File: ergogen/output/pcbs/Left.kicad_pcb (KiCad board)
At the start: 2 copper layers, 130.3 x 105.3 mm, 44 parts

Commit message: fix xiao footprint
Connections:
- MCU1 pad 17: GND -> RST
- MCU1 pad 18: RST -> GND
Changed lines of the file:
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@@
   (net 15 "DIO"))
   (pad "17" thru_hole circle (at -1.27 -6.032 90) (size 1.397 1.397) (drill 1.016) (layers "*.Cu" "*.Mask")
+  (net 17 "RST"))
+  (pad "18" thru_hole circle (at 1.27 -6.032 90) (size 1.397 1.397) (drill 1.016) (layers "*.Cu" "*.Mask")
   (net 16 "GND"))
-  (pad "18" thru_hole circle (at 1.27 -6.032 90) (size 1.397 1.397) (drill 1.016) (layers "*.Cu" "*.Mask")
-  (net 17 "RST"))
   (pad "19" thru_hole circle (at -4.445 -0.317 180) (size 1.397 1.397) (drill 1.016) (layers "*.Cu" "*.Mask")
   (net 18 "BAT"))

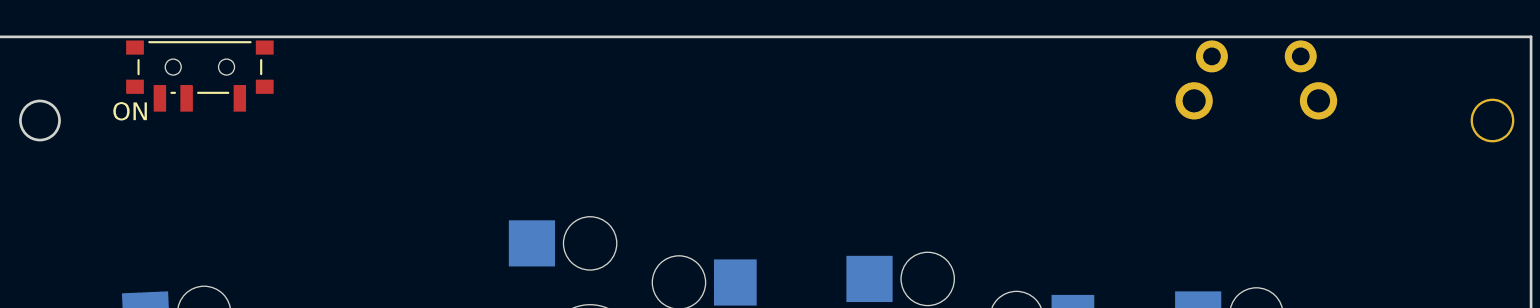
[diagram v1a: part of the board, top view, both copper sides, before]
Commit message: update config
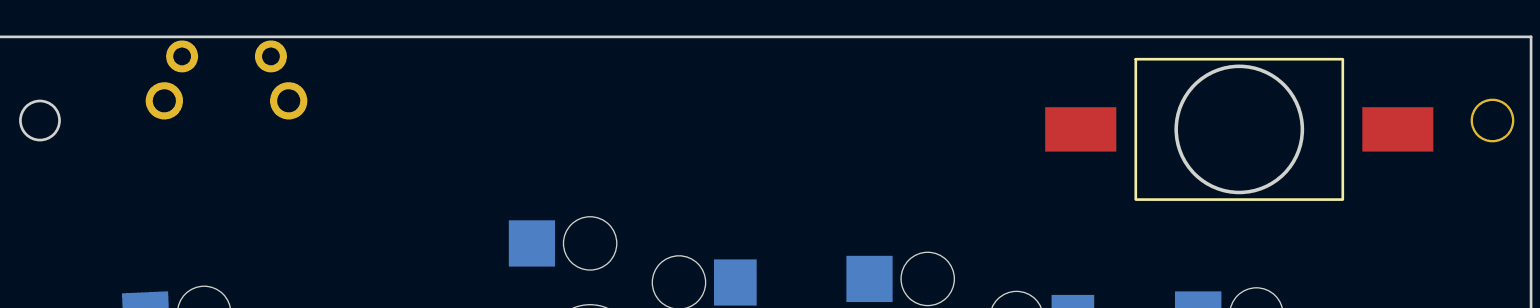
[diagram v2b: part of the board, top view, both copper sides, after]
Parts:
- SW1: footprint power_switch -> 1208YD
- moved SW1 58.6 mm to (175.2, 34.2), turned to 0 degrees
- moved S19 58.0 mm to (118.2, 31.4)
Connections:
- SW1 pad 1: (no net) -> BAT
- SW1 pad 2: BAT -> BAT_CONN
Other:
- board text removed: "ON"
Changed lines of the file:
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@@
             (pad 2 smd rect (at 1.65 0 -15) (size 0.9 1.2) (layers F.Cu F.Paste F.Mask) (net 38 "extension_cluster"))
         )
-        (module power_switch (layer F.Cu)
-          (at 116.6705308 30.73354019999999 90)
-          (attr smd)
-          (fp_text reference "SW1" (at -3.6 0 0) (layer F.SilkS) hide
-            (effects (font (size 1 1) (thickness 0.15)))
-          )
-          (fp_line (start 0.415 -3.45) (end -0.375 -3.45) (layer F.SilkS) (width 0.12))
-          (fp_line (start -0.375 3.45) (end 0.415 3.45) (layer F.SilkS) (width 0.12))
-          (fp_line (start -1.425 1.6) (end -1.425 -0.1) (layer F.SilkS) (width 0.12))
-          (fp_line (start 1.425 2.85) (end 1.425 -2.85) (layer F.SilkS) (width 0.12))
-          (fp_line (start 1.795 4.4) (end -2.755 4.4) (layer F.CrtYd) (width 0.05))
-          (fp_line (start 1.795 1.65) (end 1.795 4.4) (layer F.CrtYd) (width 0.05))
-          (fp_line (start 3.095 1.65) (end 1.795 1.65) (layer F.CrtYd) (width 0.05))
-          (fp_line (start 3.095 -1.65) (end 3.095 1.65) (layer F.CrtYd) (width 0.05))
-          (fp_line (start 1.795 -1.65) (end 3.095 -1.65) (layer F.CrtYd) (width 0.05))
-          (fp_line (start 1.795 -4.4) (end 1.795 -1.65) (layer F.CrtYd) (width 0.05))
-          (fp_line (start -2.755 -4.4) (end 1.795 -4.4) (layer F.CrtYd) (width 0.05))
-          (fp_line (start -2.755 4.4) (end -2.755 -4.4) (layer F.CrtYd) (width 0.05))
-          (fp_line (start -1.425 -1.4) (end -1.425 -1.6) (layer F.SilkS) (width 0.12))
-          (fp_line (start -1.305 -3.35) (end -1.305 3.35) (layer F.Fab) (width 0.1))
-          (fp_line (start 1.295 -3.35) (end -1.305 -3.35) (layer F.Fab) (width 0.1))
-          (fp_line (start 1.295 3.35) (end 1.295 -3.35) (layer F.Fab) (width 0.1))
-          (fp_line (start -1.305 3.35) (end 1.295 3.35) (layer F.Fab) (width 0.1))
-          (fp_line (start 2.595 0.1) (end 1.295 0.1) (layer F.Fab) (width 0.1))
-          (fp_line (start 2.645 0.15) (end 2.595 0.1) (layer F.Fab) (width 0.1))
-          (fp_line (start 2.845 0.35) (end 2.645 0.15) (layer F.Fab) (width 0.1))
-          (fp_line (start 2.845 1.2) (end 2.845 0.35) (layer F.Fab) (width 0.1))
-          (fp_line (start 2.645 1.4) (end 2.845 1.2) (layer F.Fab) (width 0.1))
-          (fp_line (start 1.345 1.4) (end 2.645 1.4) (layer F.Fab) (width 0.1))
-          (pad "" smd rect (at 1.125 -3.65 180) (size 1 0.8) (layers F.Cu F.Paste F.Mask))
-          (pad "" smd rect (at -1.085 -3.65 180) (size 1 0.8) (layers F.Cu F.Paste F.Mask))
-          (pad "" smd rect (at -1.085 3.65 180) (size 1 0.8) (layers F.Cu F.Paste F.Mask))
-          (pad 1 smd rect (at -1.735 2.25 180) (size 0.7 1.5) (layers F.Cu F.Paste F.Mask))
-          (pad 2 smd rect (at -1.735 -0.75 180) (size 0.7 1.5) (layers F.Cu F.Paste F.Mask) (net 18 "BAT"))
-          (pad 3 smd rect (at -1.735 -2.25 180) (size 0.7 1.5) (layers F.Cu F.Paste F.Mask) (net 39 "BAT_CONN"))
-          (pad "" smd rect (at 1.125 3.65 180) (size 1 0.8) (layers F.Cu F.Paste F.Mask))
-          (pad "" np_thru_hole circle (at 0.025 -1.5 180) (size 0.9 0.9) (drill 0.9) (layers *.Cu *.Mask))
-          (pad "" np_thru_hole circle (at 0.025 1.5 180) (size 0.9 0.9) (drill 0.9) (layers *.Cu *.Mask))
-        )
-      (gr_text "ON" (at 112.77053079999999 33.23354019999999 0) (layer F.SilkS)
-        (effects (font (size 1 1) (thickness 0.15)))
-      )
+(footprint "1208YD"
+  (layer "F.Cu")
+  (at 175.1705308 34.21654019999999 0)
+  (property "Reference" "SW1"
+    (at 0 -0.5 0)
+    (layer "F.SilkS")
+    hide
+    (effects (font (size 1 1) (thickness 0.1)))
+  )
+  (attr smd)
+  (fp_rect (start -5.825 -3.95) (end 5.825 3.95) (stroke (width 0.15) (type default)) (fill none) (layer "F.SilkS"))
+  (fp_circle (center 0 0) (end 3.55 0) (stroke (width 0.2) (type default)) (fill none) (layer "Edge.Cuts"))
+  (pad "1" smd rect (at -8.925 0 0) (size 4 2.5) (layers "F.Cu" "F.Paste" "F.Mask")
+    (thermal_bridge_angle 45)
+    (net 18 "BAT"))
+  (pad "2" smd rect (at 8.925 0 0) (size 4 2.5) (layers "F.Cu" "F.Paste" "F.Mask")
+    (thermal_bridge_angle 45)
+    (net 39 "BAT_CONN"))
+)
 (module "SKHLLCA010" (layer "F.Cu")
-        (at 176.13053079999997 31.35854019999999 0)
+        (at 118.1705308 31.35854019999999 0)
   (attr through_hole)
   (fp_text reference "S19" (at -2.25 3.5 0) (layer F.SilkS) hide
@@
   (fp_line (start -3.65 -4.97) (end -3.65 2.18) (layer "F.CrtYd") (width 0.05))
   (fp_line (start -3.65 2.18) (end 3.65 2.18) (layer "F.CrtYd") (width 0.05))
-  (pad "1" thru_hole circle (at 2.5 -1.25 0) (size 1.8 1.8) (drill 1) (layers *.Cu "B.Mask") (net 17 "RST"))
-  (pad "2" thru_hole circle (at -2.5 -1.25 0) (size 1.8 1.8) (drill 1) (layers *.Cu "B.Mask") (net 16 "GND"))
+  (pad "1" thru_hole circle (at -2.5 -1.25 0) (size 1.8 1.8) (drill 1) (layers *.Cu "B.Mask") (net 17 "RST"))
+  (pad "2" thru_hole circle (at 2.5 -1.25 0) (size 1.8 1.8) (drill 1) (layers *.Cu "B.Mask") (net 16 "GND"))
   (pad "MP" thru_hole circle (at -3.5 1.25 0) (size 2.1 2.1) (drill 1.3) (layers *.Cu *.Mask))
   (pad "MP" thru_hole circle (at 3.5 1.25 0) (size 2.1 2.1) (drill 1.3) (layers *.Cu *.Mask))
